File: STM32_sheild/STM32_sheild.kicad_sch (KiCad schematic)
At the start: 51 parts, among them J1 61612002121503, J2 CN7, J3 CN10, J4 632722100213, J5 691210910002, J6 691210910002, U1 OPA333xxDBV, U2 TPS63031DSK, U3 MCP73831-2-MC, U4 OPA333xxDBV

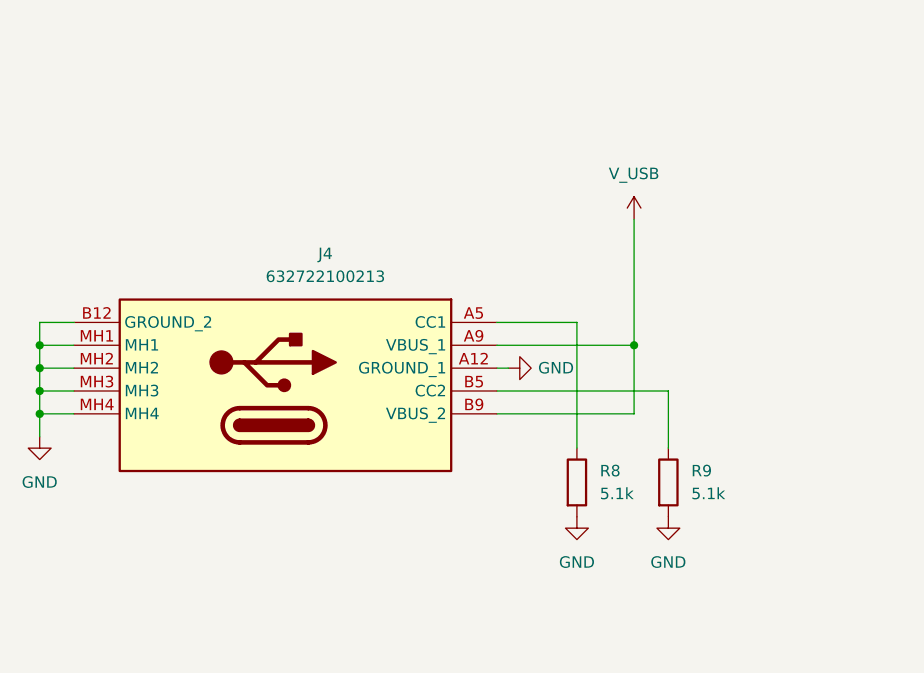
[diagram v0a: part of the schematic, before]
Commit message: update
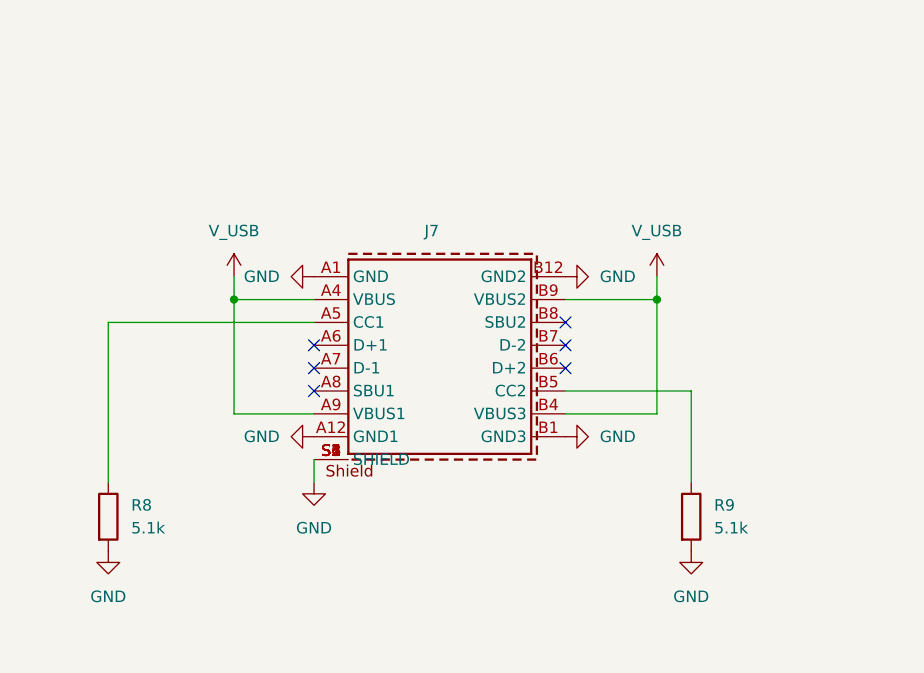
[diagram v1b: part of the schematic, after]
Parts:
- removed J4: 632722100213, KiCad_wurth_USB-C_PD_connector:632722100213, symbol 632722100213:632722100213
- added J7: 629722010114, Connector_SMD_Wurth:J_Wurth_WR-USB_629722010114, symbol Connector_Wurth_WR-USB:629722010114
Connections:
- net GND: now also J7.A1 (GND), J7.A12 (GND1), J7.B1 (GND3), J7.B12 (GND2), J7.S1 (SHIELD), J7.S2 (SHIELD), J7.S3 (SHIELD), J7.S4 (SHIELD), J7.S5 (SHIELD), J7.S6 (SHIELD)
- net V_USB: now also J7.A4 (VBUS), J7.A9 (VBUS1), J7.B4 (VBUS3), J7.B9 (VBUS2)
- net at R8.1: now also J7.A5 (CC1)
- net at R9.1: now also J7.B5 (CC2)
- no-connect marks 0 -> 6
